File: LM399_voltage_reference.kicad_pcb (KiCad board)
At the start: 2 copper layers, 72.5 x 40.5 mm, 12 parts, among them U1 LM399, U2 LTC2057

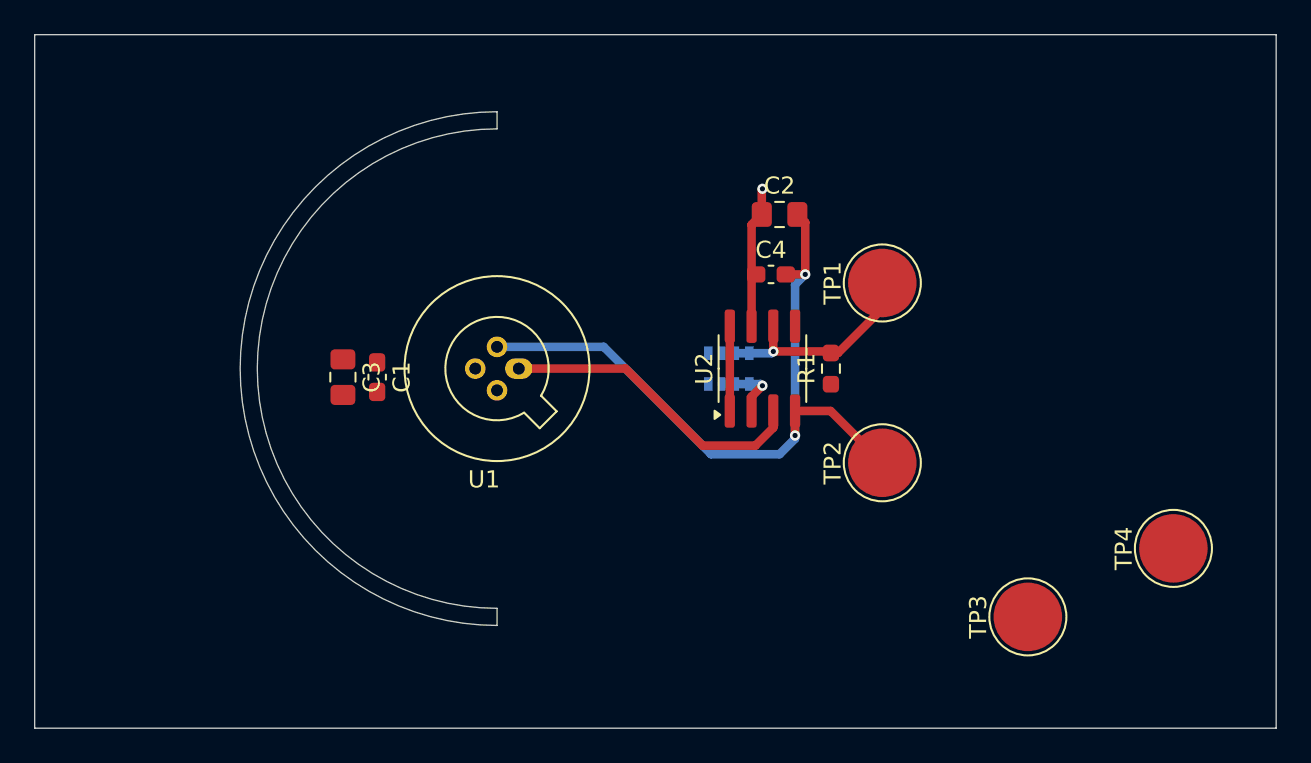
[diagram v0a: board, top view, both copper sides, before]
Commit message: Nearly there.
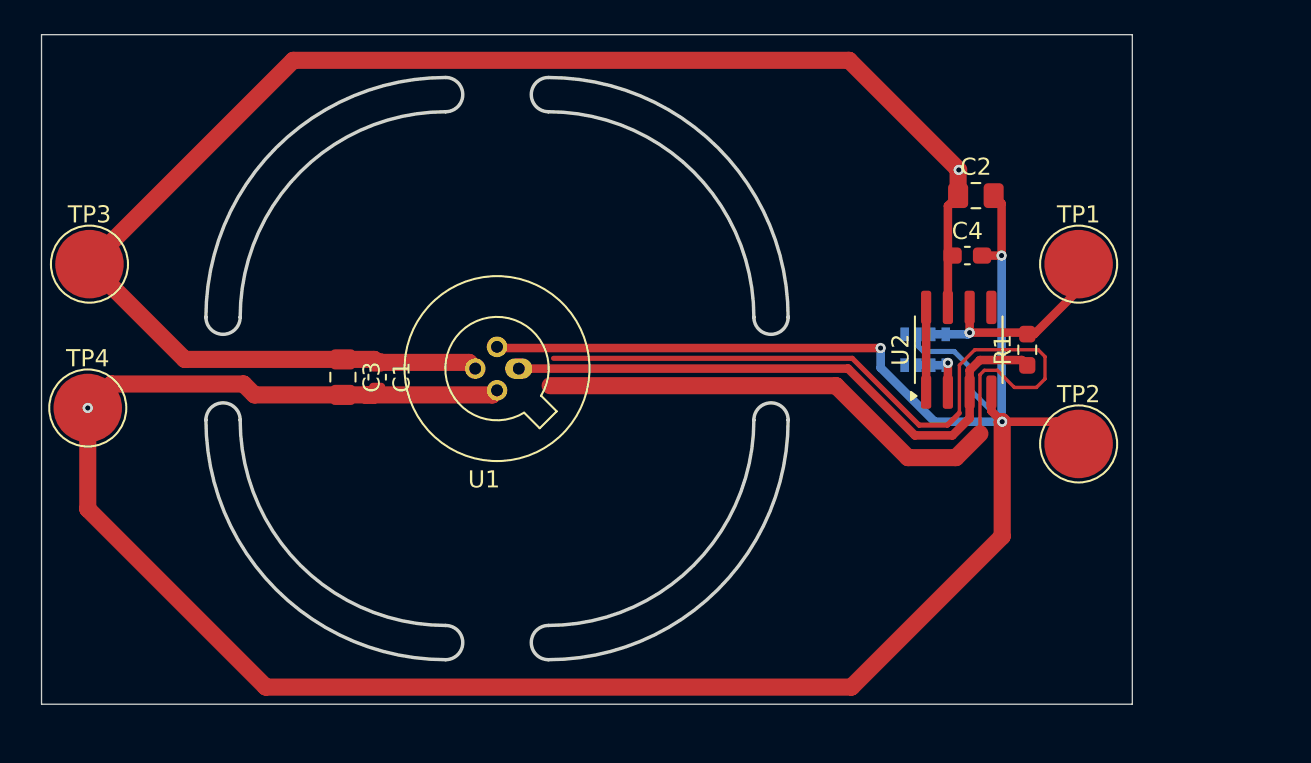
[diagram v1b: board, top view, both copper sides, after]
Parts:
- moved TP4 63.9 mm to (176.1, 102.3), turned to 0 degrees
- moved TP3 58.5 mm to (176.2, 93.9), turned to 0 degrees
- moved C2 11.5 mm to (228.0, 89.9)
- moved C4 11.5 mm to (227.5, 93.4)
- moved R1 11.5 mm to (231.0, 98.9)
- moved RN1 11.5 mm to (225.0, 98.9)
- moved TP1 11.5 mm to (234.0, 93.9), turned to 0 degrees
- moved TP2 11.5 mm to (234.0, 104.4), turned to 0 degrees
- moved U2 11.5 mm to (227.0, 98.9)
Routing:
- net GND: track 42.8 -> 161.3 mm, vias 2 -> 4
- net vcc: track 8.29 -> 91.7 mm
- net unconnected-(RN1-R4.2-Pad5): track 0.00 -> 70.7 mm
- net Net-(U2-+): track 18.1 -> 34.9 mm
- net Net-(RN1-R1.1): track 4.14 -> 3.49 mm
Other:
- board size 72.5 x 40.5 mm -> 63.7 x 39.1 mm
